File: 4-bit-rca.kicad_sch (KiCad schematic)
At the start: 25 parts, among them J1 Cin, J2 Cout, SW1 SW_SPST, SW2 SW_SPST, SW3 SW_SPST, SW4 SW_SPST, SW5 SW_SPST, SW6 SW_SPST, SW7 SW_SPST, SW8 SW_SPST, U1 74HC86, U2 74HC08, U3 74HC32, U4 74HC08, U5 74HC86, U6 L7805

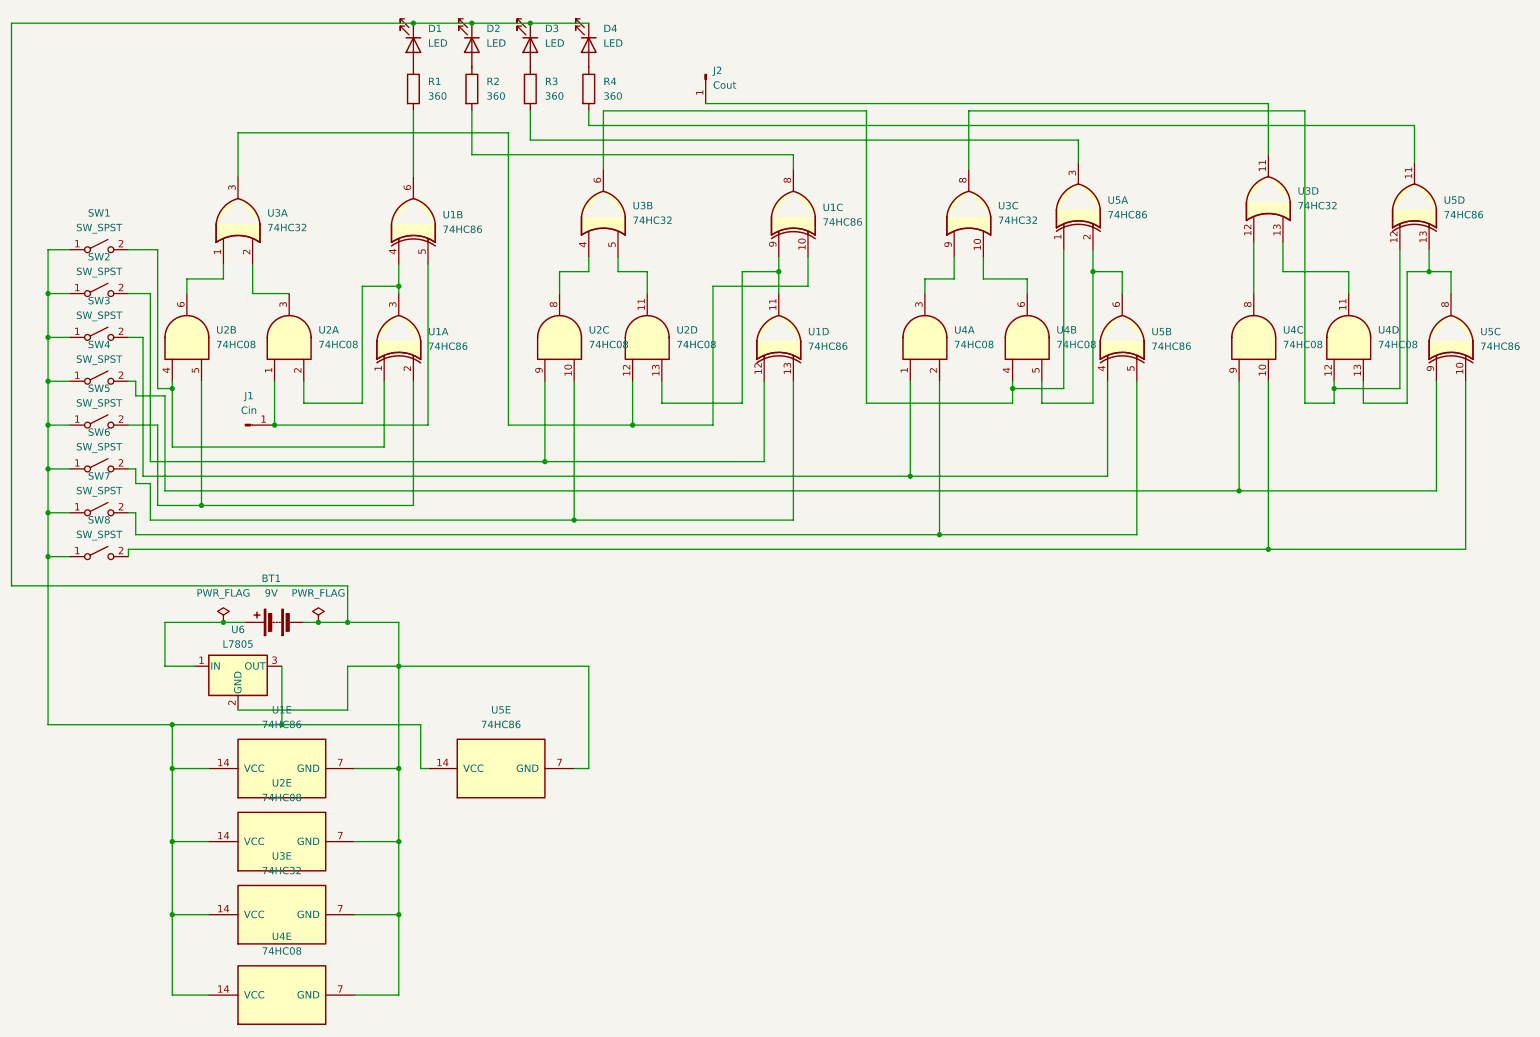
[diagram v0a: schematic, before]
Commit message: aoisjdojoasd
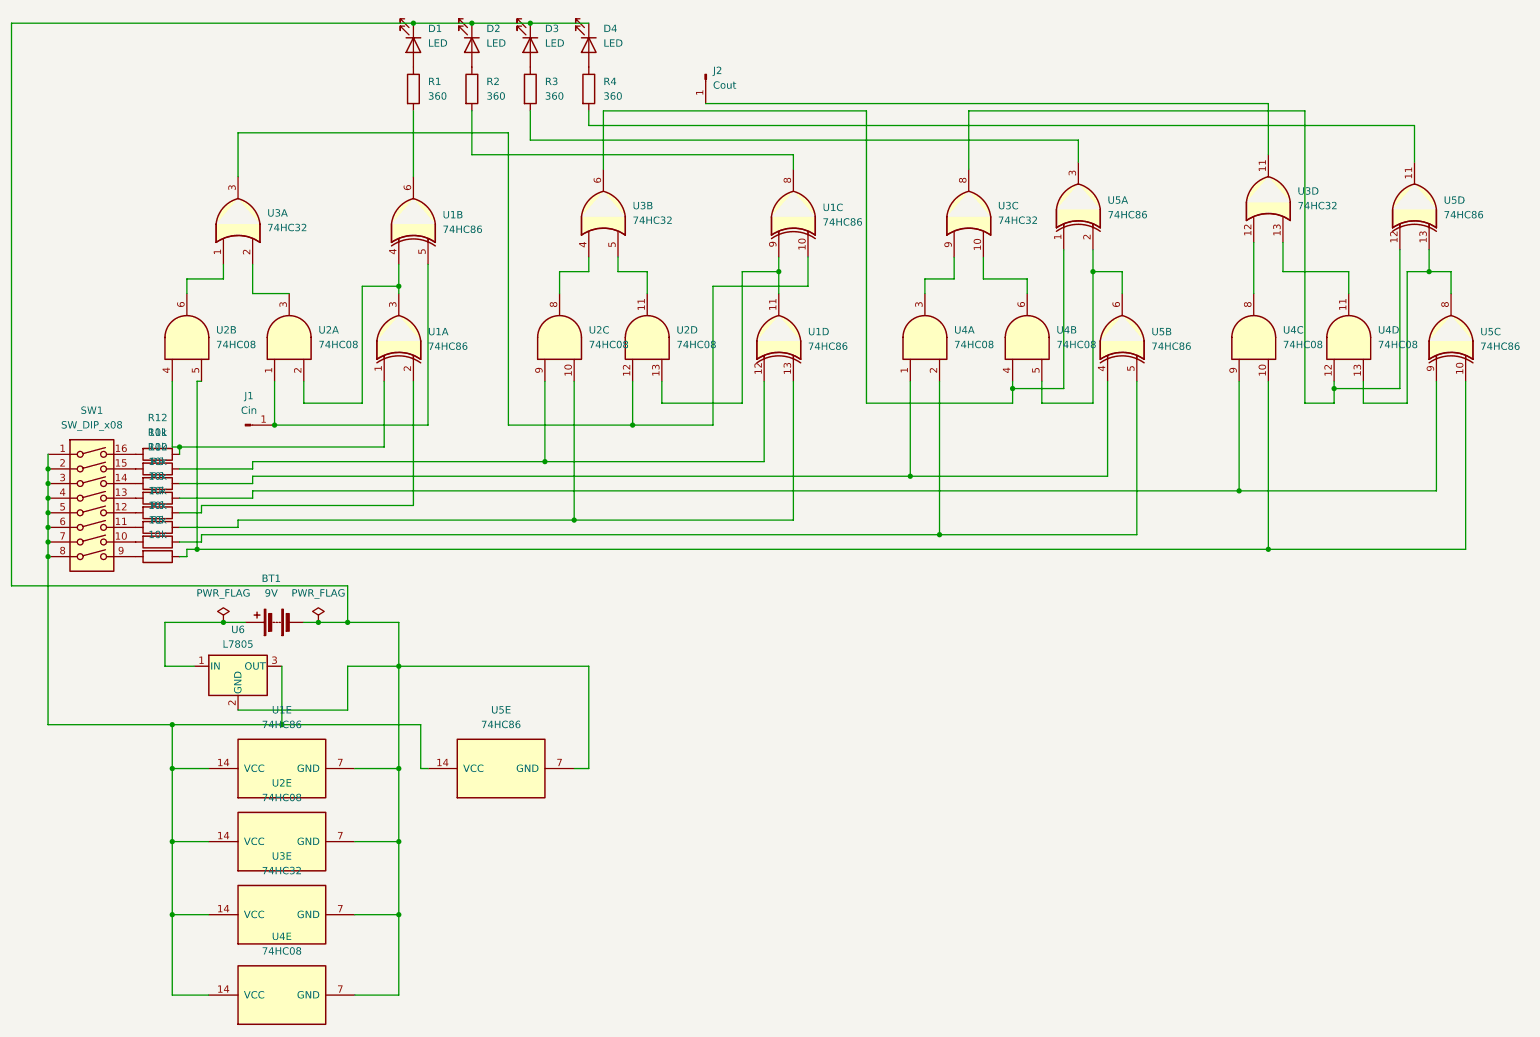
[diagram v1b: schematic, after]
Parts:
- removed SW1, SW2, SW3, SW4, SW5, SW6, SW7, SW8: SW_SPST, Button_Switch_THT:SW_PUSH_6mm, symbol Switch:SW_SPST
- added R10, R11, R12, R5, R6, R7, R8, R9: 10k, Resistor_THT:R_Axial_DIN0207_L6.3mm_D2.5mm_P10.16mm_Horizontal, symbol Device:R
- added SW1: SW_DIP_x08, Button_Switch_SMD:SW_DIP_SPSTx08_Slide_9.78x22.5mm_W8.61mm_P2.54mm, symbol Switch:SW_DIP_x08
- U6: footprint Package_TO_SOT_THT:TO-92 -> Package_TO_SOT_THT:TO-220-3_Vertical
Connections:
- net at U1.14 (VCC), U2.14 (VCC), U3.14 (VCC)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: now also SW1.1, SW1.2, SW1.3, SW1.4, SW1.5, SW1.6, SW1.7, SW1.8
- net at U4.1, U5.4: now also R10.1
- net at U4.2, U5.5: now also R6.1
- net at U1.1, U2.4: now also R12.1
- net at U2.5: now also U4.10, U5.10, R5.1; no longer U1.2
- net at U4.9, U5.9: now also R9.1
- net at U1.13, U2.10: now also R7.1
- net at U1.12, U2.9: now also R11.1
- new net: R7.2, SW1.11
- new net: R6.2, SW1.10
- new net: R8.2, SW1.12
- new net: R9.2, SW1.13
- new net: R10.2, SW1.14
- new net: R11.2, SW1.15
- new net: R12.2, SW1.16
- new net: R5.2, SW1.9
- new net: R8.1, U1.2

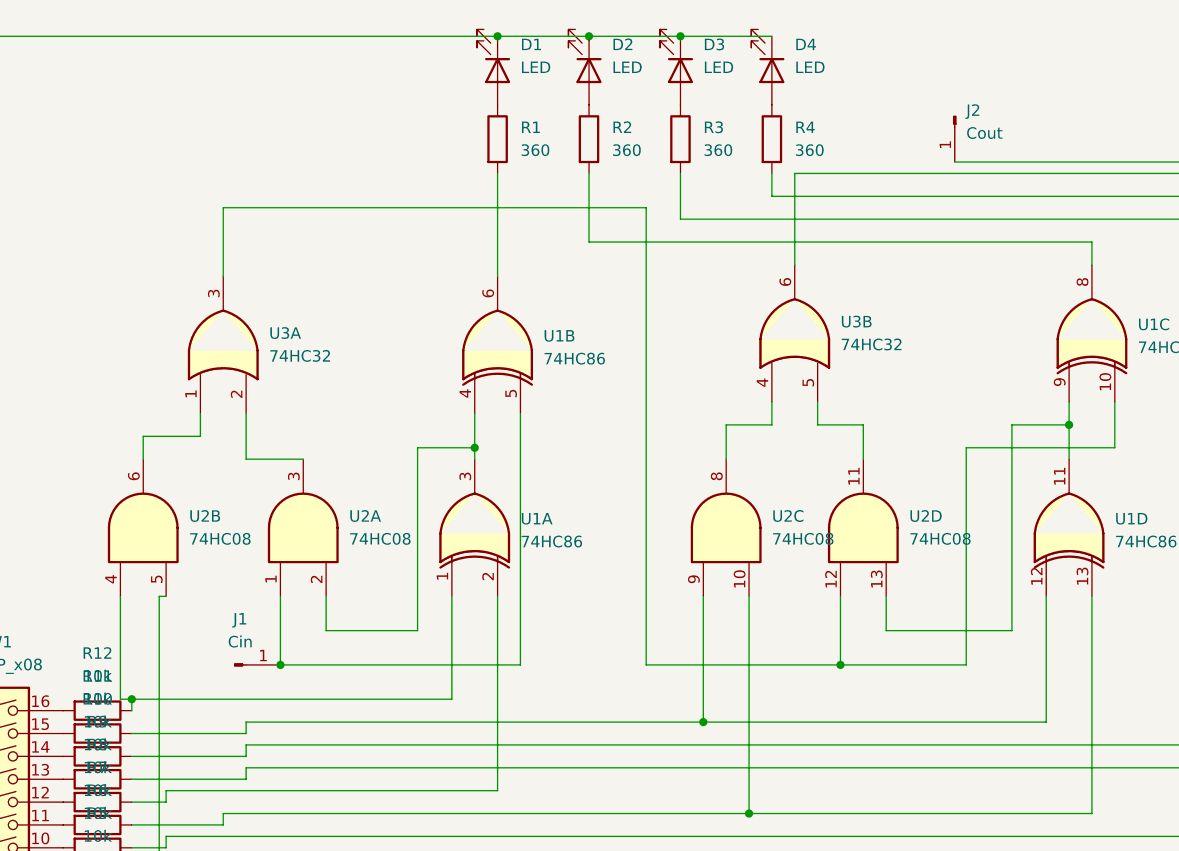
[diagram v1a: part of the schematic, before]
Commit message: a
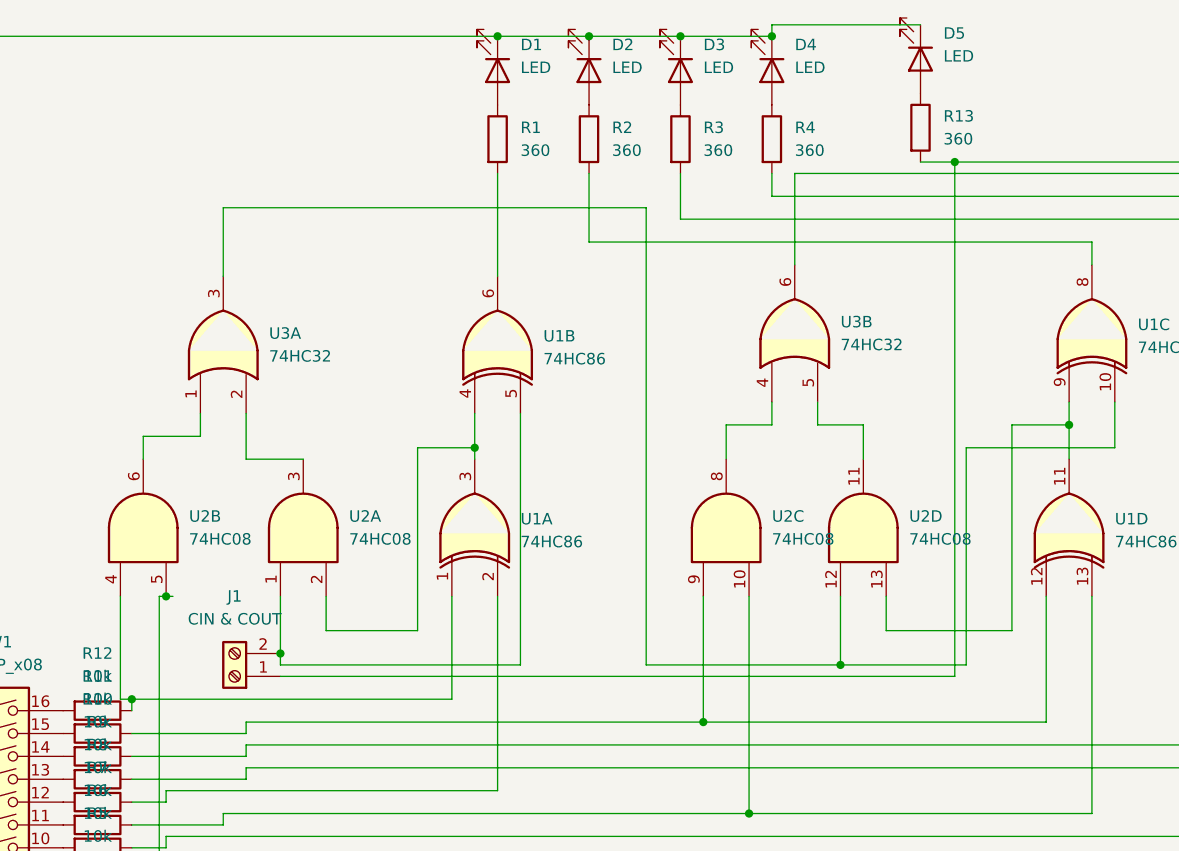
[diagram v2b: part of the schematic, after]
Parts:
- removed J1: Cin, Connector_PinHeader_2.54mm:PinHeader_1x01_P2.54mm_Vertical, symbol Connector:Conn_01x01_Pin
- removed J2: Cout, Connector_PinHeader_2.54mm:PinHeader_1x01_P2.54mm_Vertical, symbol Connector:Conn_01x01_Pin
- added D5: LED, LED_THT:LED_D5.0mm, symbol Device:LED
- added J1: CIN & COUT, Connector_PinHeader_2.54mm:PinHeader_1x02_P2.54mm_Vertical, symbol Connector:Screw_Terminal_01x02
- added R13: 360, Resistor_THT:R_Axial_DIN0207_L6.3mm_D2.5mm_P10.16mm_Horizontal, symbol Device:R
- SW1: footprint Button_Switch_SMD:SW_DIP_SPSTx08_Slide_9.78x22.5mm_W8.61mm_P2.54mm -> Button_Switch_THT:SW_DIP_SPSTx08_Slide_6.7x21.88mm_W7.62mm_P2.54mm_LowProfile
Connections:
- net at BT1.2 (-), D1.1 (K), D2.1 (K)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: now also D5.1 (K)
- net at U1.5, U2.1: now also J1.2 (Pin_2)
- net at U3.11: now also J1.1 (Pin_1), R13.2
- new net: D5.2 (A), R13.1
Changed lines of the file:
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@@
   (junction (at 25.4 102.87) (diameter 0) (color 0 0 0 0)
   )
+  (junction (at 64.77 83.82) (diameter 0) (color 0 0 0 0)
+  )
+  (junction (at 139.7 29.21) (diameter 0) (color 0 0 0 0)
+  )
   (junction (at 86.36 60.96) (diameter 0) (color 0 0 0 0)
   )
+  (junction (at 119.38 15.24) (diameter 0) (color 0 0 0 0)
+  )
   (junction (at 193.04 78.74) (diameter 0) (color 0 0 0 0)
   )
@@
   (junction (at 88.9 15.24) (diameter 0) (color 0 0 0 0)
   )
+  (junction (at 52.07 77.47) (diameter 0) (color 0 0 0 0)
+  )
   (junction (at 25.4 92.71) (diameter 0) (color 0 0 0 0)
   )
@@
   (junction (at 248.92 78.74) (diameter 0) (color 0 0 0 0)
   )
-  (junction (at 64.77 85.09) (diameter 0) (color 0 0 0 0)
-  )
   (junction (at 111.76 91.44) (diameter 0) (color 0 0 0 0)
   )
@@
     (stroke (width 0) (type default))
   )
+  (wire (pts (xy 139.7 86.36) (xy 139.7 29.21))
+    (stroke (width 0) (type default))
+  )
   (wire (pts (xy 48.26 102.87) (xy 58.42 102.87))
     (stroke (width 0) (type default))
@@
     (stroke (width 0) (type default))
   )
+  (wire (pts (xy 119.38 13.97) (xy 119.38 15.24))
+    (stroke (width 0) (type default))
+  )
   (wire (pts (xy 99.06 15.24) (xy 88.9 15.24))
     (stroke (width 0) (type default))
@@
     (stroke (width 0) (type default))
   )
+  (wire (pts (xy 52.832 77.47) (xy 52.07 77.47))
+    (stroke (width 0) (type default))
+  )
   (wire (pts (xy 204.47 35.56) (xy 109.22 35.56))
     (stroke (width 0) (type default))
@@
     (stroke (width 0) (type default))
   )
+  (wire (pts (xy 64.77 86.36) (xy 139.7 86.36))
+    (stroke (width 0) (type default))
+  )
   (wire (pts (xy 55.88 119.38) (xy 59.69 119.38))
     (stroke (width 0) (type default))
@@
     (stroke (width 0) (type default))
   )
+  (wire (pts (xy 135.89 29.21) (xy 139.7 29.21))
+    (stroke (width 0) (type default))
+  )
   (wire (pts (xy 212.09 58.42) (xy 207.01 58.42))
     (stroke (width 0) (type default))
   )
+  (wire (pts (xy 64.77 83.82) (xy 64.77 85.09))
+    (stroke (width 0) (type default))
+  )
   (wire (pts (xy 77.47 127) (xy 86.36 127))
     (stroke (width 0) (type default))
@@
     (stroke (width 0) (type default))
   )
-  (wire (pts (xy 64.77 77.47) (xy 64.77 85.09))
+  (wire (pts (xy 64.77 77.47) (xy 64.77 83.82))
+    (stroke (width 0) (type default))
+  )
+  (wire (pts (xy 135.89 13.97) (xy 119.38 13.97))
     (stroke (width 0) (type default))
   )
@@
     (stroke (width 0) (type default))
   )
+  (symbol (lib_id "Device:R") (at 135.89 25.4 0) (unit 1)
+    (in_bom yes) (on_board yes) (dnp no) (fields_autoplaced)
+    (property "Reference" "R13" (at 138.43 24.13 0)
+      (effects (font (size 1.27 1.27)) (justify left))
+    )
+    (property "Value" "360" (at 138.43 26.67 0)
+      (effects (font (size 1.27 1.27)) (justify left))
+    )
+    (property "Footprint" "Resistor_THT:R_Axial_DIN0207_L6.3mm_D2.5mm_P10.16mm_Horizontal" (at 134.112 25.4 90)
+      (effects (font (size 1.27 1.27)) hide)
+    )
+    (property "Datasheet" "~" (at 135.89 25.4 0)
+      (effects (font (size 1.27 1.27)) hide)
+    )
+    (pin "1")
+    (pin "2")
+    (instances
+      (project "4-bit-rca"
+        (path "/efee30f6-5335-4726-a007-a60c5d8e691f"
+          (reference "R13") (unit 1)
+        )
+      )
+    )
+  )
   (symbol (lib_id "74xx:74LS86") (at 66.04 144.78 90) (unit 5)
     (in_bom yes) (on_board yes) (dnp no) (fields_autoplaced)
@@
       (effects (font (size 1.27 1.27)))
     )
-    (property "Footprint" "Button_Switch_SMD:SW_DIP_SPSTx08_Slide_9.78x22.5mm_W8.61mm_P2.54mm" (at 33.02 100.33 0)
+    (property "Footprint" "Button_Switch_THT:SW_DIP_SPSTx08_Slide_6.7x21.88mm_W7.62mm_P2.54mm_LowProfile" (at 33.02 100.33 0)
       (effects (font (size 1.27 1.27)) hide)
     )
@@
     )
   )
-  (symbol (lib_id "Connector:Conn_01x01_Pin") (at 59.69 85.09 0) (unit 1)
-    (in_bom yes) (on_board yes) (dnp no) (fields_autoplaced)
-    (property "Reference" "J1" (at 60.325 80.01 0)
-      (effects (font (size 1.27 1.27)))
-    )
-    (property "Value" "Cin" (at 60.325 82.55 0)
-      (effects (font (size 1.27 1.27)))
-    )
-    (property "Footprint" "Connector_PinHeader_2.54mm:PinHeader_1x01_P2.54mm_Vertical" (at 59.69 85.09 0)
-      (effects (font (size 1.27 1.27)) hide)
-    )
-    (property "Datasheet" "~" (at 59.69 85.09 0)
-      (effects (font (size 1.27 1.27)) hide)
-    )
-    (pin "1")
-    (instances
-      (project "4-bit-rca"
-        (path "/efee30f6-5335-4726-a007-a60c5d8e691f"
-          (reference "J1") (unit 1)
-        )
-      )
-    )
-  )
   (symbol (lib_id "Device:LED") (at 99.06 19.05 270) (unit 1)
     (in_bom yes) (on_board yes) (dnp no) (fields_autoplaced)
@@
     )
   )
+  (symbol (lib_id "Device:LED") (at 135.89 17.78 270) (unit 1)
+    (in_bom yes) (on_board yes) (dnp no) (fields_autoplaced)
+    (property "Reference" "D5" (at 138.43 14.9225 90)
+      (effects (font (size 1.27 1.27)) (justify left))
+    )
+    (property "Value" "LED" (at 138.43 17.4625 90)
+      (effects (font (size 1.27 1.27)) (justify left))
+    )
+    (property "Footprint" "LED_THT:LED_D5.0mm" (at 135.89 17.78 0)
+      (effects (font (size 1.27 1.27)) hide)
+    )
+    (property "Datasheet" "~" (at 135.89 17.78 0)
+      (effects (font (size 1.27 1.27)) hide)
+    )
+    (pin "2")
+    (pin "1")
+    (instances
+      (project "4-bit-rca"
+        (path "/efee30f6-5335-4726-a007-a60c5d8e691f"
+          (reference "D5") (unit 1)
+        )
+      )
+    )
+  )
+  (symbol (lib_id "Connector:Screw_Terminal_01x02") (at 59.69 86.36 180) (unit 1)
+    (in_bom yes) (on_board yes) (dnp no) (fields_autoplaced)
+    (property "Reference" "J1" (at 59.69 77.47 0)
+      (effects (font (size 1.27 1.27)))
+    )
+    (property "Value" "CIN & COUT" (at 59.69 80.01 0)
+      (effects (font (size 1.27 1.27)))
+    )
+    (property "Footprint" "Connector_PinHeader_2.54mm:PinHeader_1x02_P2.54mm_Vertical" (at 59.69 86.36 0)
+      (effects (font (size 1.27 1.27)) hide)
+    )
+    (property "Datasheet" "~" (at 59.69 86.36 0)
+      (effects (font (size 1.27 1.27)) hide)
+    )
+    (pin "1")
+    (pin "2")
+    (instances
+      (project "4-bit-rca"
+        (path "/efee30f6-5335-4726-a007-a60c5d8e691f"
+          (reference "J1") (unit 1)
+        )
+      )
+    )
+  )
   (symbol (lib_id "74xx:74LS08") (at 234.95 69.85 90) (unit 3)
     (in_bom yes) (on_board yes) (dnp no) (fields_autoplaced)
@@
         )
       )
-    )
-  )
-  (symbol (lib_id "Connector:Conn_01x01_Pin") (at 139.7 24.13 270) (unit 1)
-    (in_bom yes) (on_board yes) (dnp no) (fields_autoplaced)
-    (property "Reference" "J2" (at 140.97 23.495 90)
-      (effects (font (size 1.27 1.27)) (justify left))
-    )
-    (property "Value" "Cout" (at 140.97 26.035 90)
-      (effects (font (size 1.27 1.27)) (justify left))
-    )
-    (property "Footprint" "Connector_PinHeader_2.54mm:PinHeader_1x01_P2.54mm_Vertical" (at 139.7 24.13 0)
-      (effects (font (size 1.27 1.27)) hide)
-    )
-    (property "Datasheet" "~" (at 139.7 24.13 0)
-      (effects (font (size 1.27 1.27)) hide)
-    )
-    (pin "1")
-    (instances
-      (project "4-bit-rca"
-        (path "/efee30f6-5335-4726-a007-a60c5d8e691f"
-          (reference "J2") (unit 1)
-        )
-      )
